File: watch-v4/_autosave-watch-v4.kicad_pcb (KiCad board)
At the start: 4 copper layers, 13 x 35 mm, 38 parts, among them J1 CONN_10, P1 Expansion Header, Q1 MOSFET_P, U1 IC_MCP73831, U2 MAX1722, U3 DS3231, U4 LSM9DS0, U5 NRF51822, U6 BALUN, X1 16mhz

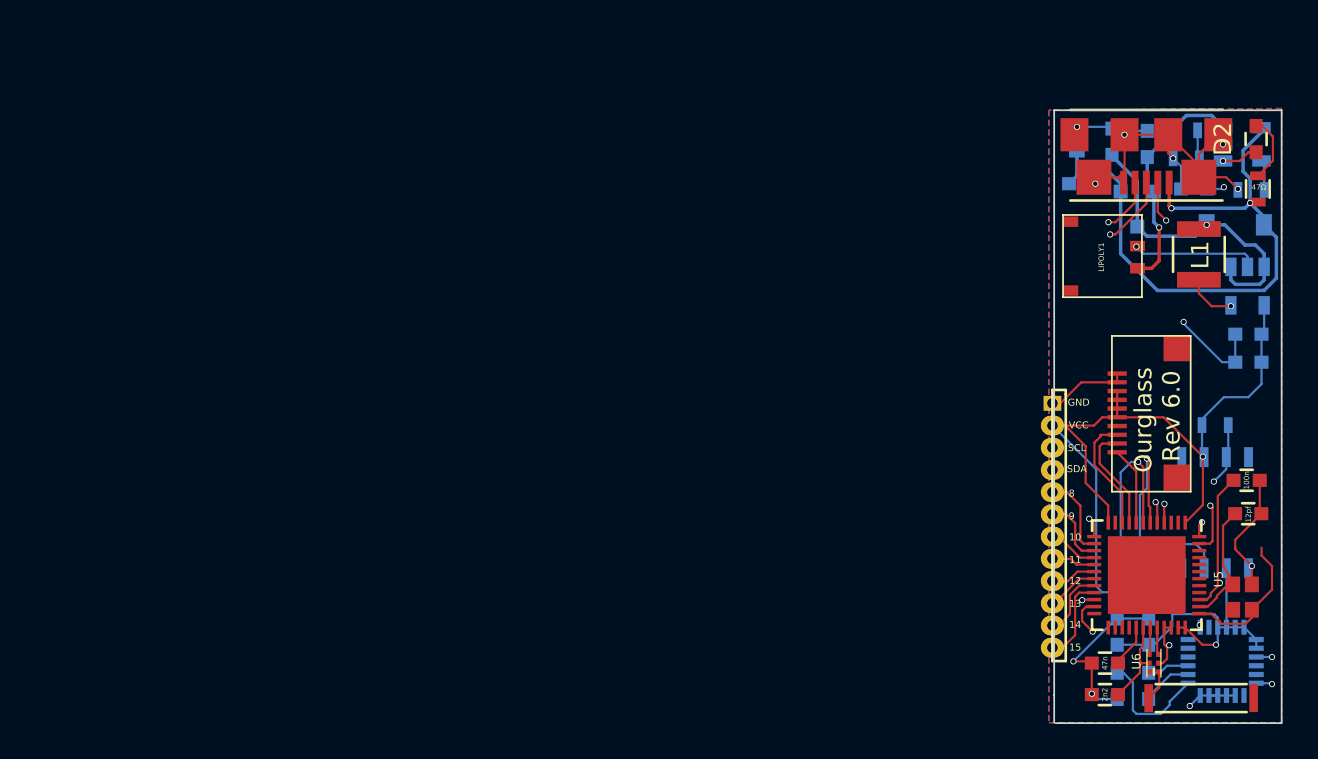
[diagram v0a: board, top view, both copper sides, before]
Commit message: v6 as sent to fab (errors!)
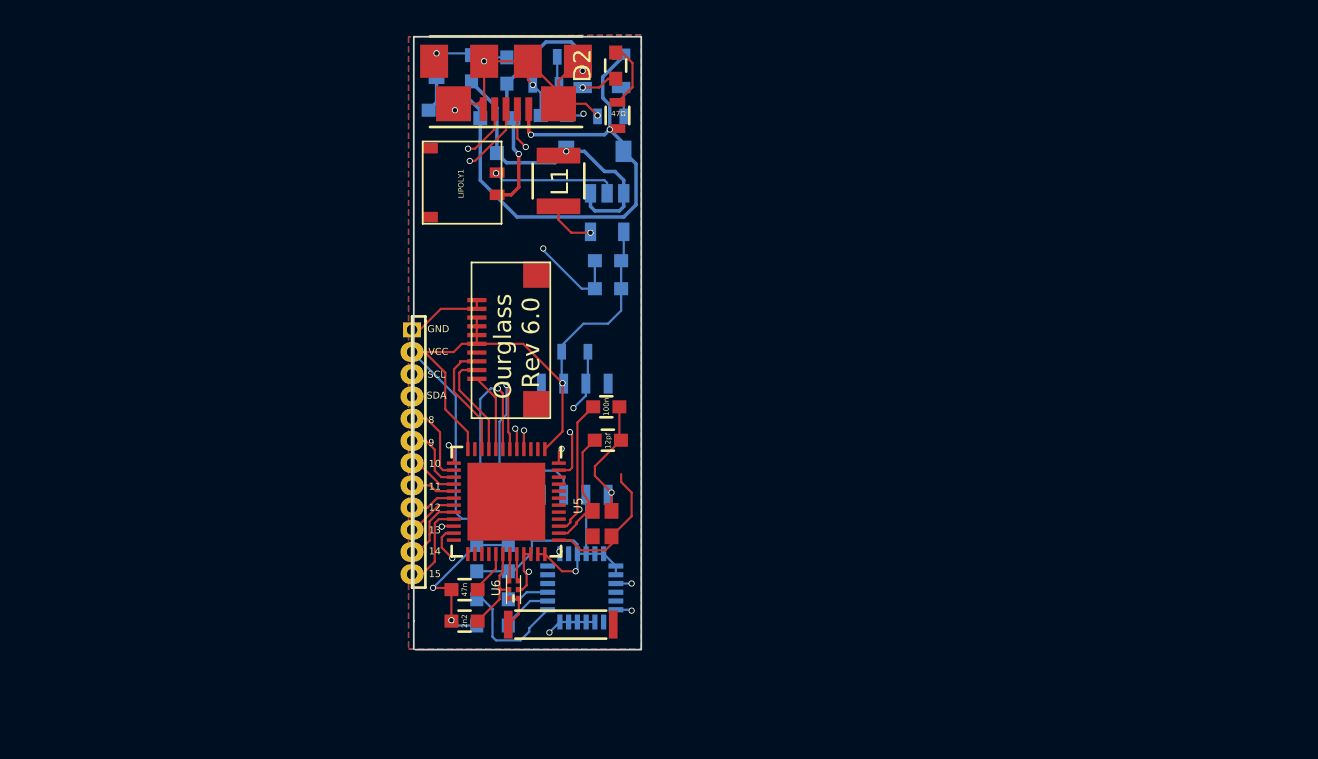
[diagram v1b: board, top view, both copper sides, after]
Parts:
- moved C13 36.8 mm to (146.7, 90.9)
- moved C14 36.8 mm to (146.7, 89.3)
- moved C2 36.8 mm to (137.2, 80.7)
- moved C3 36.8 mm to (140.9, 78.4)
- moved C6 36.8 mm to (139.2, 109.4)
- moved C7 36.8 mm to (139.2, 106.3)
- moved D1 36.8 mm to (145.9, 83.0)
- moved D2 36.8 mm to (147.1, 78.2)
- moved J1 36.8 mm to (140.2, 93.8)
- moved R5 36.8 mm to (141.2, 103.4)
- moved U4 36.8 mm to (145.2, 108.0)
- moved U5 36.8 mm to (140.9, 103.1)
- moved ANT1 36.8 mm to (144.0, 110.1)
- moved C1 36.8 mm to (138.9, 78.3)
- moved C10 36.8 mm to (146.7, 99.6)
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
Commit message: v6.5
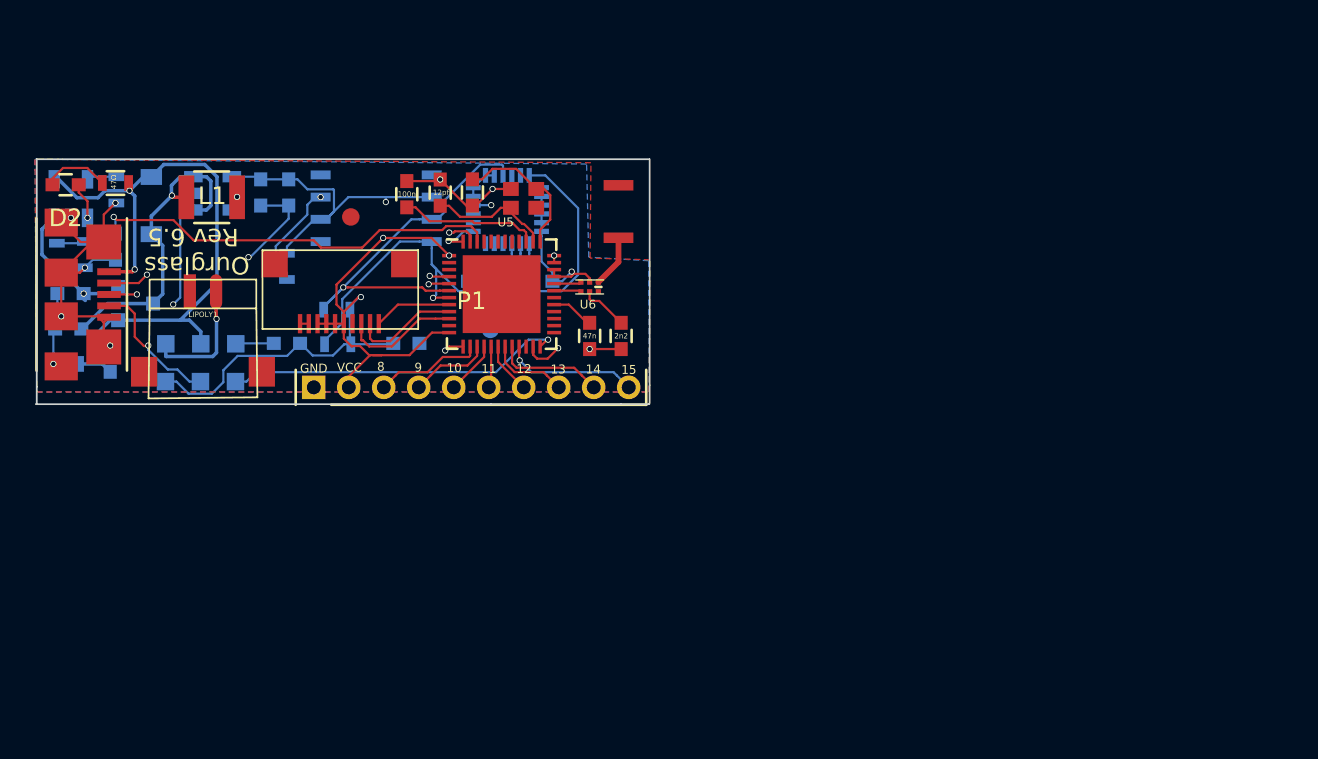
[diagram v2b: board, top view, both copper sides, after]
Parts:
- added C15: 12pf, Capacitors_SMD:C_0603, F.Cu at (138.9, 85.4)
- added P2: Test Points, crennelated:test_points, B.Cu at (123.4, 95.1)
- added REF**: F2, Fiducials:Fiducial_1mm_Dia_2.54mm_Outer_CopperTop, B.Cu at (140.0, 93.2)
- added REF**: F1, Fiducials:Fiducial_1mm_Dia_2.54mm_Outer_CopperTop, F.Cu at (132.0, 86.8)
- C6: value 4u7 -> 4.7uf
- LIPOLY1: footprint Socket_Strips:molex_2_pos -> crennelated:JST_2_pos
- P1: footprint Socket_Strips:Socket_Strip_Straight_1x12_small -> Pin_Header_Straight_1x10_Pitch2.00mm
- moved D2 32.2 mm to (115.7, 85.0), turned to 180 degrees
- moved U1 31.2 mm to (116.0, 85.8), turned to 90 degrees
- moved R7 30.1 mm to (115.2, 89.0), turned to 90 degrees
- moved R1 28.9 mm to (118.5, 84.9), turned to 0 degrees
- moved R2 28.6 mm to (118.6, 85.2), turned to 270 degrees
- moved R8 28.1 mm to (116.8, 89.0), turned to 270 degrees
- moved C3 28.0 mm to (116.0, 91.2), turned to 180 degrees
- moved C1 27.4 mm to (115.8, 93.2), turned to 180 degrees
- moved R3 27.1 mm to (115.8, 95.2), turned to 180 degrees
- moved XL1 27.1 mm to (116.6, 91.2), turned to 270 degrees
- moved C12 26.1 mm to (118.5, 88.5), turned to 270 degrees
- moved D1 25.5 mm to (120.6, 86.2), turned to 270 degrees
- moved ANT1 23.9 mm to (147.3, 86.5), turned to 90 degrees
- moved C2 23.7 mm to (118.2, 94.9), turned to 90 degrees
- moved Q1 22.8 mm to (119.7, 91.8), turned to 90 degrees
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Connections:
- C11 pad 1: /VDD_PA -> Net-(C11-Pad1)
- P1 pad 10: /EX13 -> /EX15
- P1 pad 3: /SCL -> /EX8
- P1 pad 4: /SDA -> /EX9
- P1 pad 5: /EX8 -> /EX10
- P1 pad 6: /EX9 -> /EX11
- P1 pad 7: /EX10 -> /EX12
- P1 pad 8: /EX11 -> /EX13
- P1 pad 9: /EX12 -> /EX14
- U5 pad 22: /BatterySense -> Net-(U5-Pad22)
- U5 pad 24: Net-(U5-Pad24) -> /SWDCLK
- U5 pad 30: /VDD_PA -> Net-(U5-Pad30)
- U5 pad 46: Net-(U5-Pad46) -> /BatterySense
- U6 pad 5: /VDD_PA -> Net-(C11-Pad1)
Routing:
- net /SWDCLK: track 0.00 -> 19.5 mm, vias 0 -> 1
- net /BatterySense: track 41.7 -> 27.3 mm, vias 2 -> 1
- net /SCL: track 35.9 -> 22.5 mm, vias 2 -> 1
- net /VCC: track 66.4 -> 79.2 mm, vias 2 -> 6
- net GND: track 82.2 -> 69.6 mm, vias 14 -> 13
- net /VBAT: track 13.3 -> 24.3 mm, vias 1 -> 2
- net /ClockINT: track 7.92 -> 16.7 mm
- net /SDA: track 36.3 -> 30.6 mm, vias 2 -> 1
- net /VDD_PA: track 5.13 -> 0.00 mm
- net /Reset: track 29.1 -> 33.8 mm
- net Net-(C6-Pad1): track 6.80 -> 2.22 mm
- net /Accel_INT: track 7.06 -> 2.64 mm, vias 2 -> 1
- net Net-(C11-Pad1): track 0.00 -> 2.78 mm
- net /EX15: track 5.16 -> 7.67 mm, vias 0 -> 1
- net /EXTVCC: track 35.4 -> 37.6 mm
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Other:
- board size 13 x 35 mm -> 35.1 x 14 mm
- net class 50ohm added: clearance 0.127, trace_width 0.33, via_dia 0.355, via_drill 0.254
- board text added: "Ourglass Rev 6.5"
- board text removed: "10"
- board text removed: "11"
- board text removed: "12"
- board text removed: "13"
- board text removed: "14"
- board text removed: "15"
- board text removed: "8"
- board text removed: "9"
- board text removed: "GND"
- board text removed: "Ourglass Rev 6.0"
- board text removed: "SCL"
- board text removed: "SDA"
- board text removed: "VCC"
